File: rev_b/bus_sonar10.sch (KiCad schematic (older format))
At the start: 36 parts, among them J1 TERMINATE_JUMPER, SW1 MJTP1243, U1 74HCT08, U2 LM2940, U3 MCP2562, U4 ATMEGA328_DIP28, U5 74HCT32, X1 16MHz

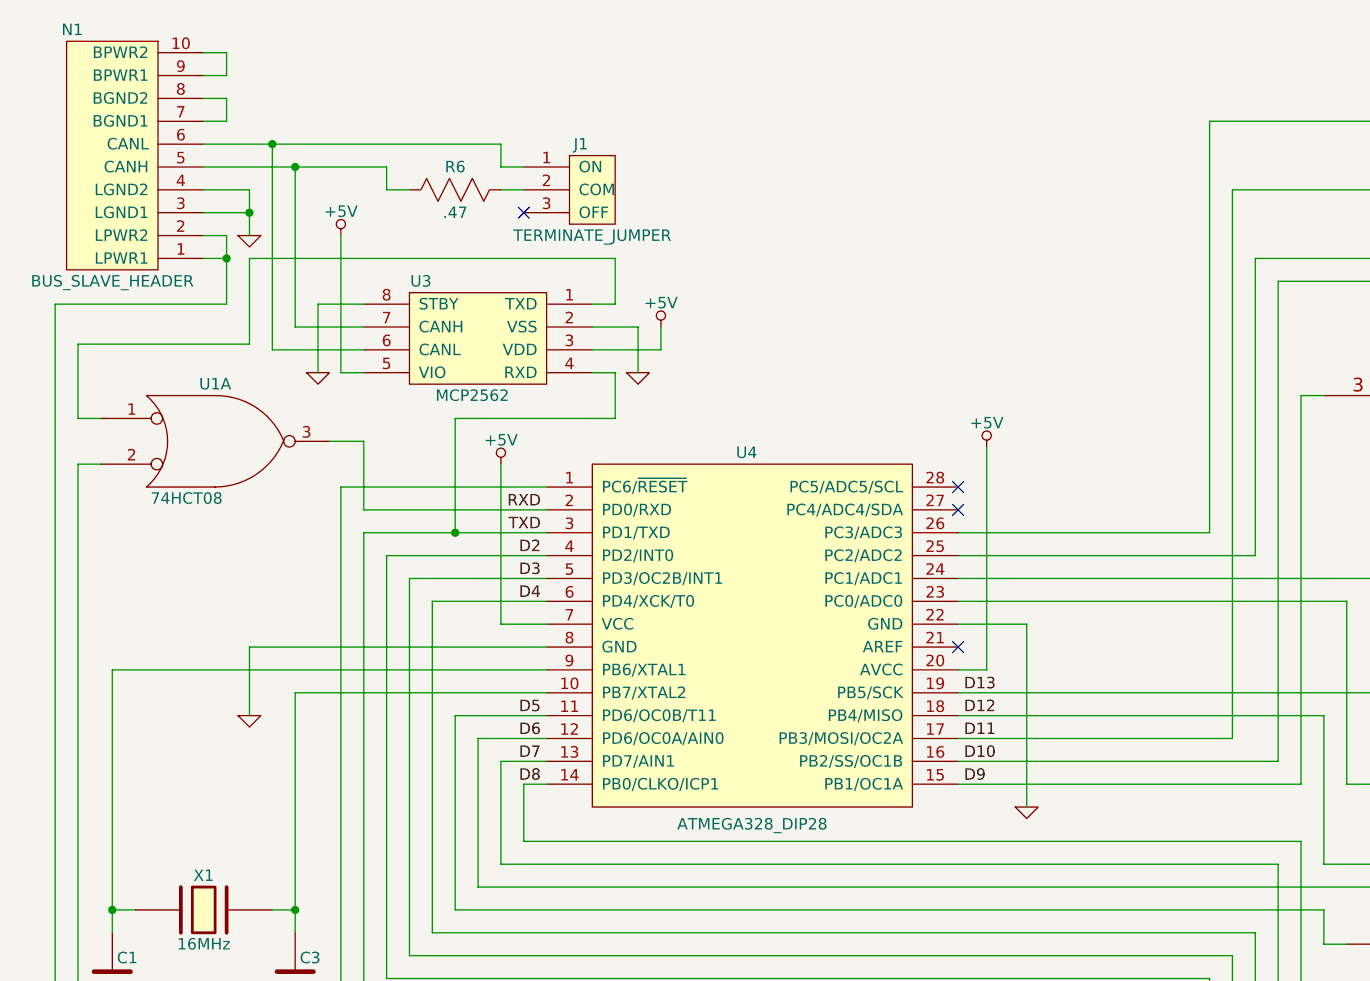
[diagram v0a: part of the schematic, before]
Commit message: Got Rev. B in pretty good shape.
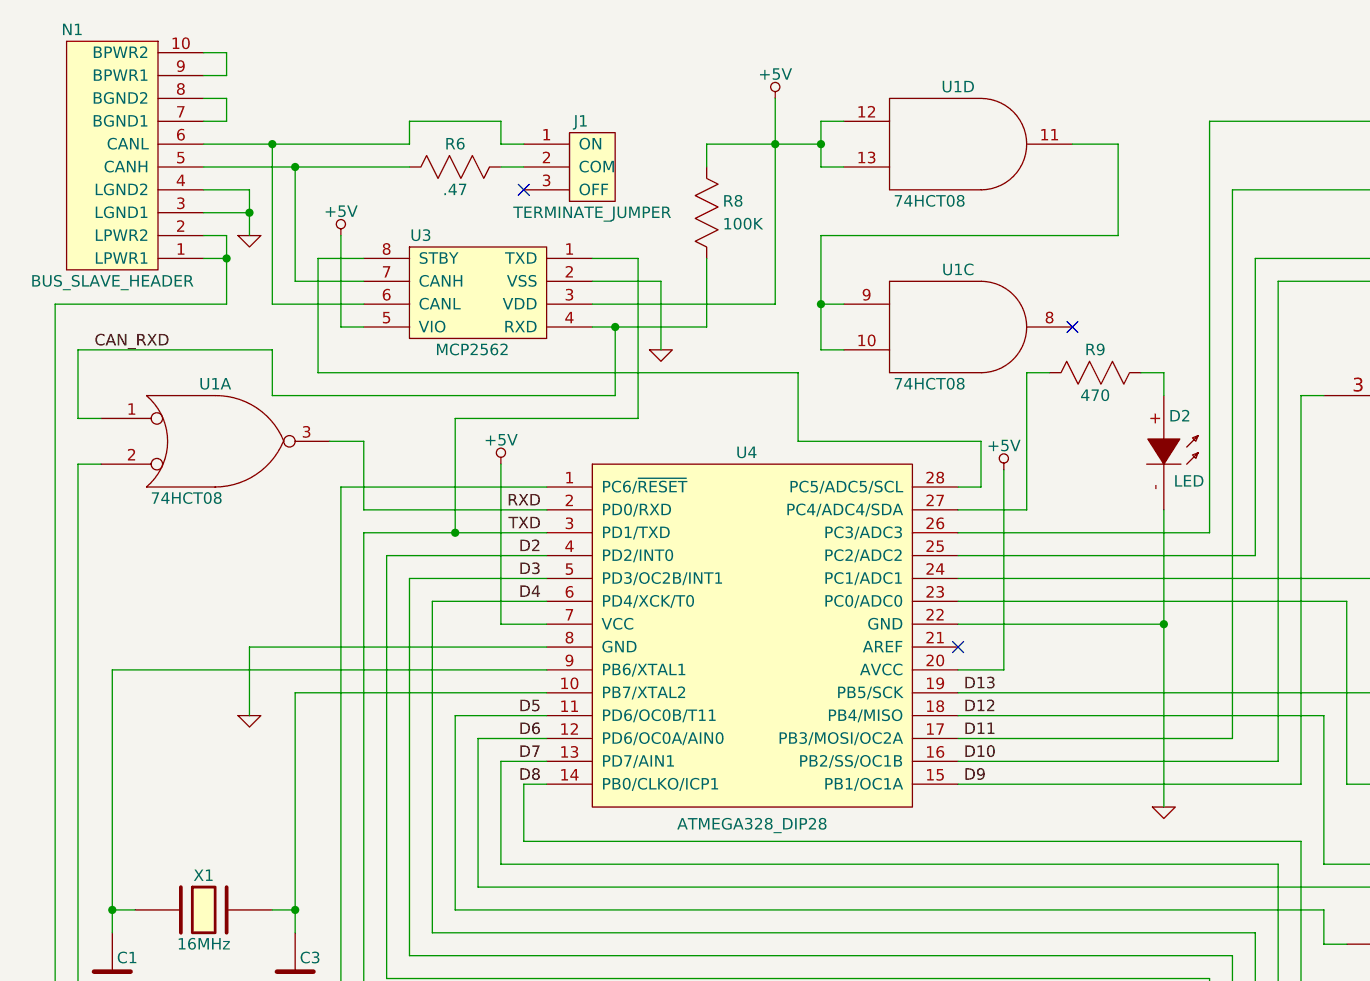
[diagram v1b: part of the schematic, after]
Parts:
- added D2: LED, bus_sonar10:T1_LED, symbol LED
- added R8: 100K, bus_sonar10:Resistor_Horizontal_400, symbol R_VERT
- added R9: 470, bus_sonar10:Resistor_Horizontal_400, symbol R_HORIZ
- added unit 4 of U1
- added unit 3 of U1
- C1, C10, C11, C3, C4, C6, C7, C8, C9: footprint (none) -> bus_sonar10:Capacitor3MMDiscRM2.5
- C2, C5: footprint (none) -> bus_sonar10:Capacitor4x3RM2-5_RevB
- D1: footprint (none) -> bus_sonar10:Diode_DO-41_SOD81_Horizontal_RM10
- G1: footprint (none) -> bus_sonar10:OSHW_LOGO_400mil
- H1, H2, H3, H4: footprint (none) -> bus_sonar10:MountingHole_3mm
- J1: footprint (none) -> bus_sonar10:Pin_Header_Straight_1x03
- N1: footprint (none) -> bus_sonar10:Pin_Header_Straight_2x05_Shrouded
- N2: footprint (none) -> bus_sonar10:Pin_Header_Straight_1x06
- N3, N4: footprint (none) -> bus_sonar10:Pin_Header_Straight_2x20_Shrouded
- R1, R2, R3, R4, R5, R6, R7: footprint (none) -> bus_sonar10:Resistor_Horizontal_400
- SW1: footprint (none) -> bus_sonar10:Button_6.5MM
- U1, U5: footprint (none) -> bus_sonar10:DIP-14__300
- U2: footprint (none) -> bus_sonar10:TO-220_Neutral123_Horizontal_LargePads
- U3: footprint (none) -> bus_sonar10:DIP-8__300
- U4: footprint (none) -> bus_sonar10:DIP-28__300
- X1: footprint (none) -> bus_sonar10:Crystal_HC49-U_Vertical
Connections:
- net +5V: now also R8.2, U1.12, U1.13, U1.14 (VCC), U1.14 (VCC)
- net GND: now also D2.-, U1.7 (GND), U1.7 (GND); no longer U3.8 (STBY)
- net TXD: now also U3.1 (TXD); no longer U3.4 (RXD)
- net at U4.27 (PC4/ADC4/SDA): now also R9.1
- net at U4.28 (PC5/ADC5/SCL): now also U3.8 (STBY)
- net CAN_RXD: now reaches U1.1
- net CAN_RXD: now also U3.4 (RXD), R8.1; no longer U3.1 (TXD)
- new net: U1.10, U1.11, U1.9
- new net: D2.+, R9.2
- no-connect marks 6 -> 5
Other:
- moved on the sheet: J1, R6, U3
